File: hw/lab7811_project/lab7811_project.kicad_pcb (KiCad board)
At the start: 2 copper layers, 41 parts, among them J1 Conn_01x06, J2 JTAG, J3 Conn_01x08_Pin, SW1 Start, SW3 Up, SW4 Reset, SW5 Down, SW6 Left, SW7 Right, U1 MPU-6050, U2 TM4C123GH6PMIR, U4 LP2950-33LPRE3, U5 Adafruit ST7735R, Y1 ABM3-16.000MHZ-B2-T

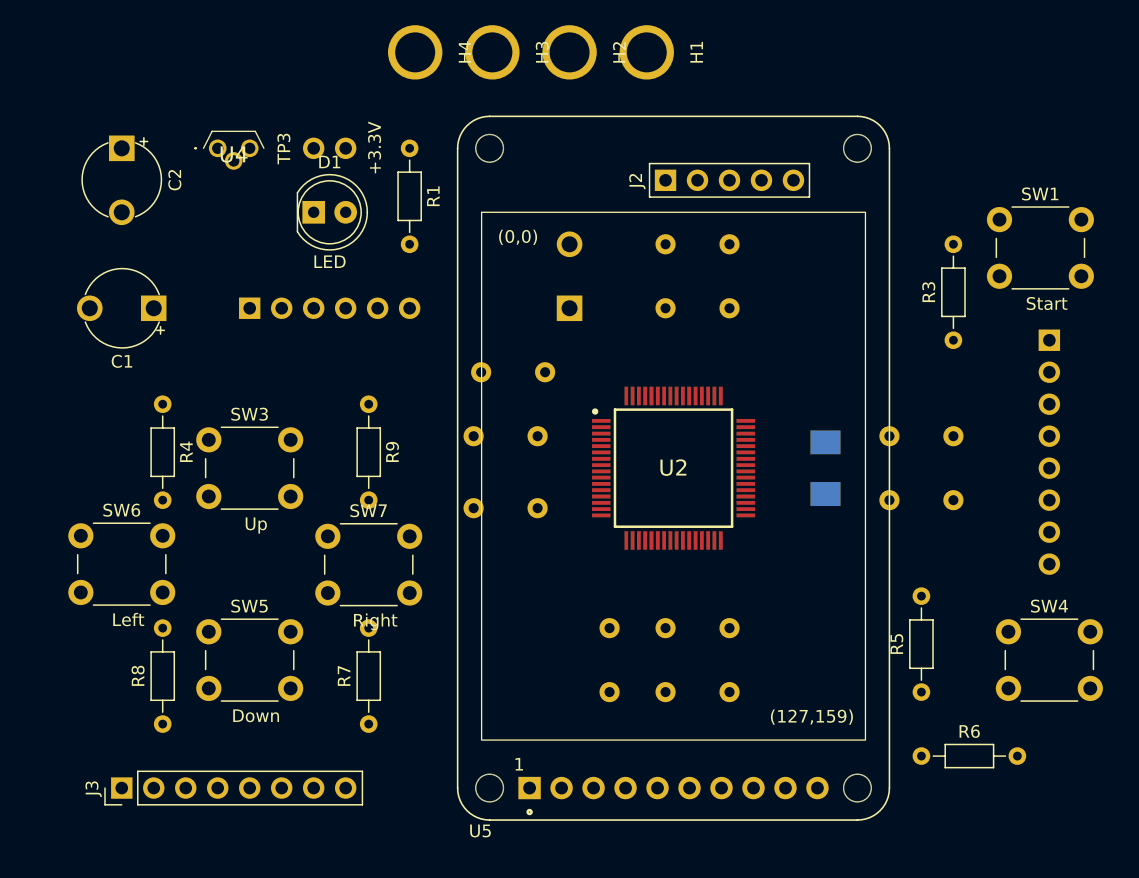
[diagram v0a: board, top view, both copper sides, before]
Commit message: finished schematic and pcb for TA review
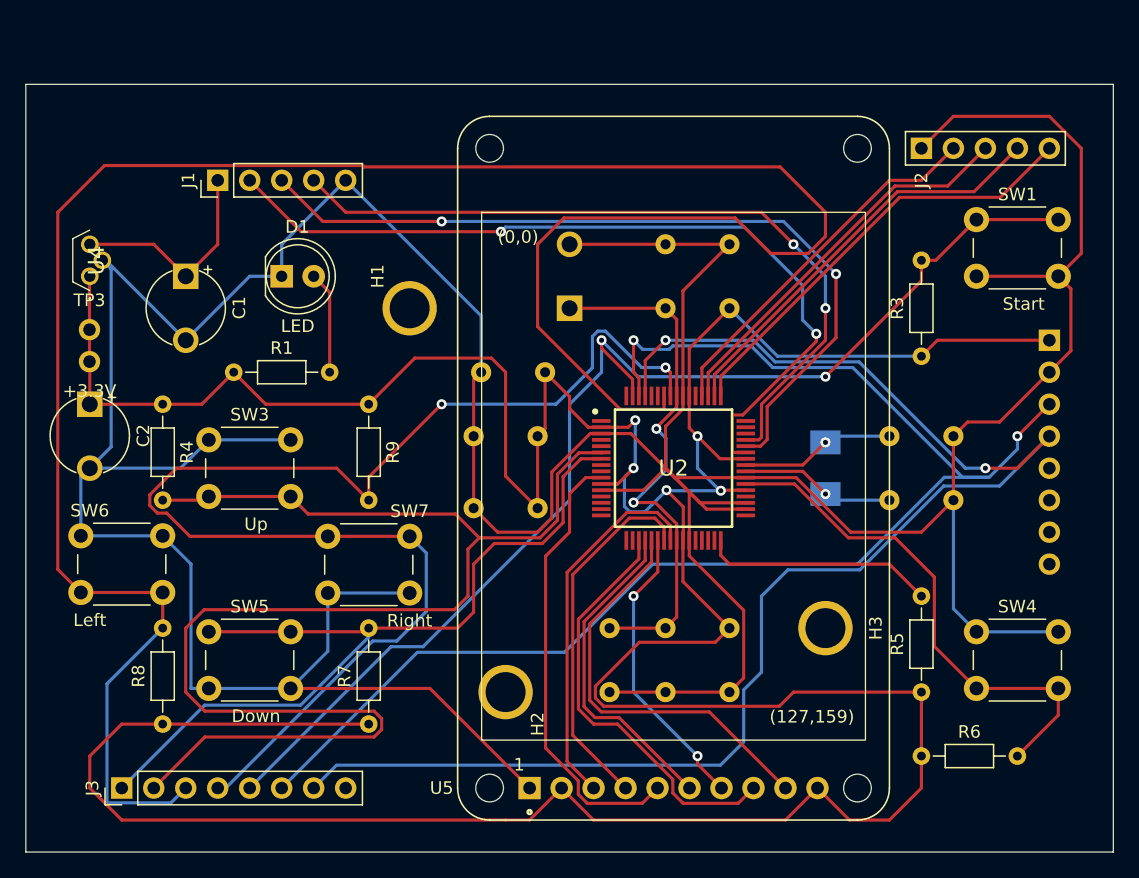
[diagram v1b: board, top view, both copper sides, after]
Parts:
- removed H4: ~, ECE445L:MountingHole_4_40
- J1: value Conn_01x06 -> Conn_01x05; footprint Connector_PinHeader_2.54mm:PinHeader_1x06_P2.54mm_Vertical -> Connector_PinHeader_2.54mm:PinHeader_1x05_P2.54mm_Vertical; moved to F.Cu
- moved H3 52.8 mm to (165.1, 91.4)
- moved H2 51.1 mm to (139.7, 96.5)
- moved H1 27.7 mm to (132.1, 66.0)
- moved TP3 22.9 mm to (106.7, 67.7), turned to 0 degrees
- moved R1 22.6 mm to (118.1, 71.1), turned to 0 degrees
- moved C2 20.5 mm to (106.7, 73.7)
- moved J2 20.5 mm to (172.7, 53.3)
- moved U4 14.4 mm to (106.7, 63.5), turned to 90 degrees
- moved J1 10.5 mm to (116.8, 55.9), turned to 90 degrees
- moved D1 5.68 mm to (121.9, 63.5)
- moved C1 3.59 mm to (114.3, 63.5), turned to -90 degrees
- moved R3 2.84 mm to (172.7, 69.8)
- moved SW4 2.54 mm to (177.1, 91.7)
- moved SW1 1.83 mm to (177.1, 59.0)
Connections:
- J1 pad 2: GND -> PD4
- J1 pad 3: PE4 -> PD5
- J1 pad 4: PE5 -> PB0
- J1 pad 5: unconnected-(J1-RTS-Pad5) -> GND
- J3 pad 3: PE4 -> PB4
- J3 pad 4: PE5 -> PB5
- R3 pad 1: +3.3V -> +3V3
- R4 pad 1: +3.3V -> +3V3
- R7 pad 1: +3.3V -> +3V3
- R8 pad 1: +3.3V -> +3V3
- R9 pad 1: +3.3V -> +3V3
- U1 pad 13: +3.3V -> +3V3
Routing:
- net GND: track 1.12 -> 368.5 mm
- net +3V3: track 0.00 -> 308.6 mm, vias 0 -> 5
- net PB4: track 0.00 -> 174.5 mm
- net PD0: track 0.00 -> 116.8 mm, vias 0 -> 2
- net PE3: track 0.00 -> 112.1 mm
- net PD1: track 0.00 -> 111.8 mm, vias 0 -> 2
- net PB5: track 0.00 -> 106.0 mm, vias 0 -> 2
- net PD2: track 0.00 -> 97.7 mm, vias 0 -> 2
- net PE2: track 0.00 -> 66.5 mm
- net PD4: track 0.00 -> 65.7 mm, vias 0 -> 2
- net PD5: track 0.00 -> 64.4 mm, vias 0 -> 2
- net PB0: track 0.00 -> 60.0 mm, vias 0 -> 2
- net /LDO: track 0.00 -> 42.7 mm, vias 0 -> 2
- net /Reset: track 0.00 -> 41.5 mm
- net PD7: track 0.00 -> 35.9 mm
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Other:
- board outline added: 86.4 x 61 mm
